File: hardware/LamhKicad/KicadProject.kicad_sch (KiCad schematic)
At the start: 45 parts, among them J1 JTAG-10 PIN, J2 436500303, J3 436500303, J4 436500303, J5 ESQ-110-X-X-D, J6 436500303, U1 TJA1051T-3, U2 PCA9685PW_112, U3 TLV70433DBVT, U4 STM32F072C8Tx

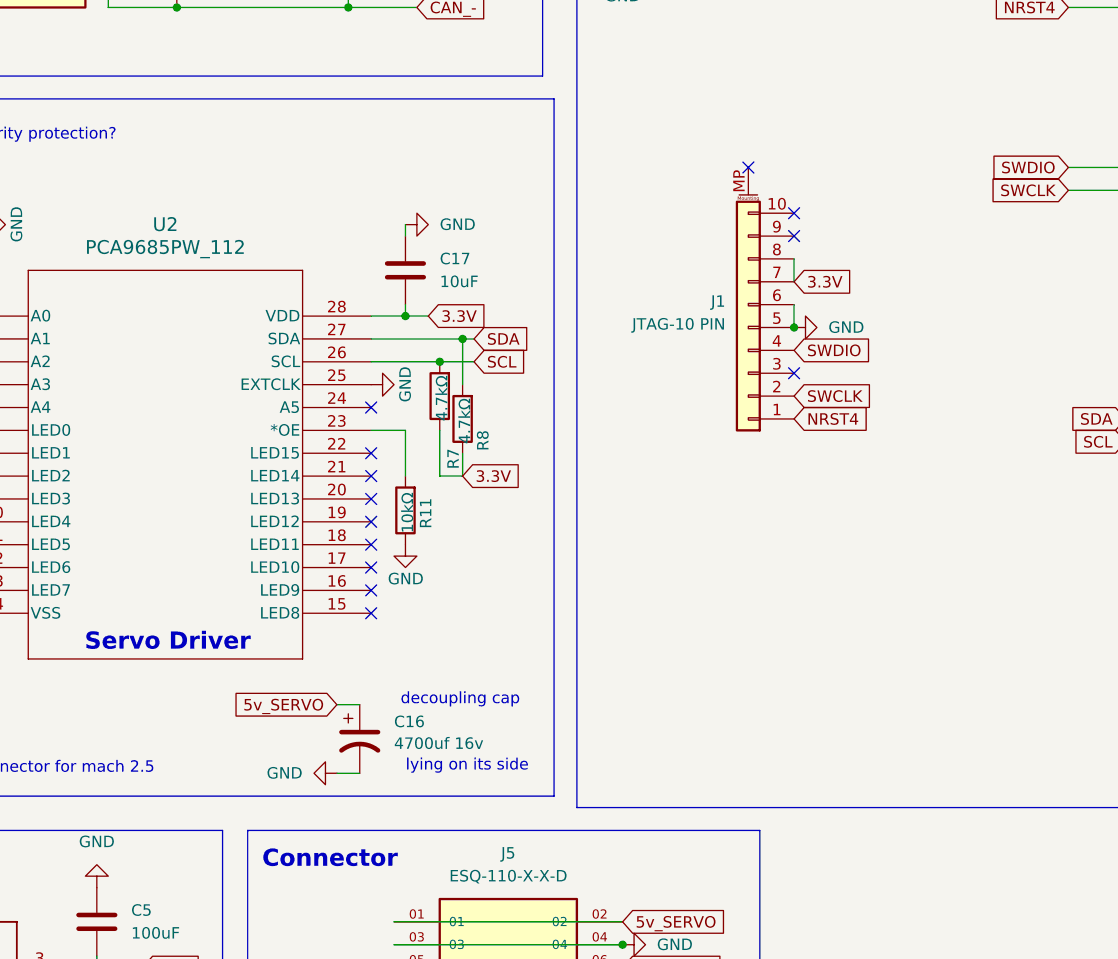
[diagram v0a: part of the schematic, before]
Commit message: ready to route
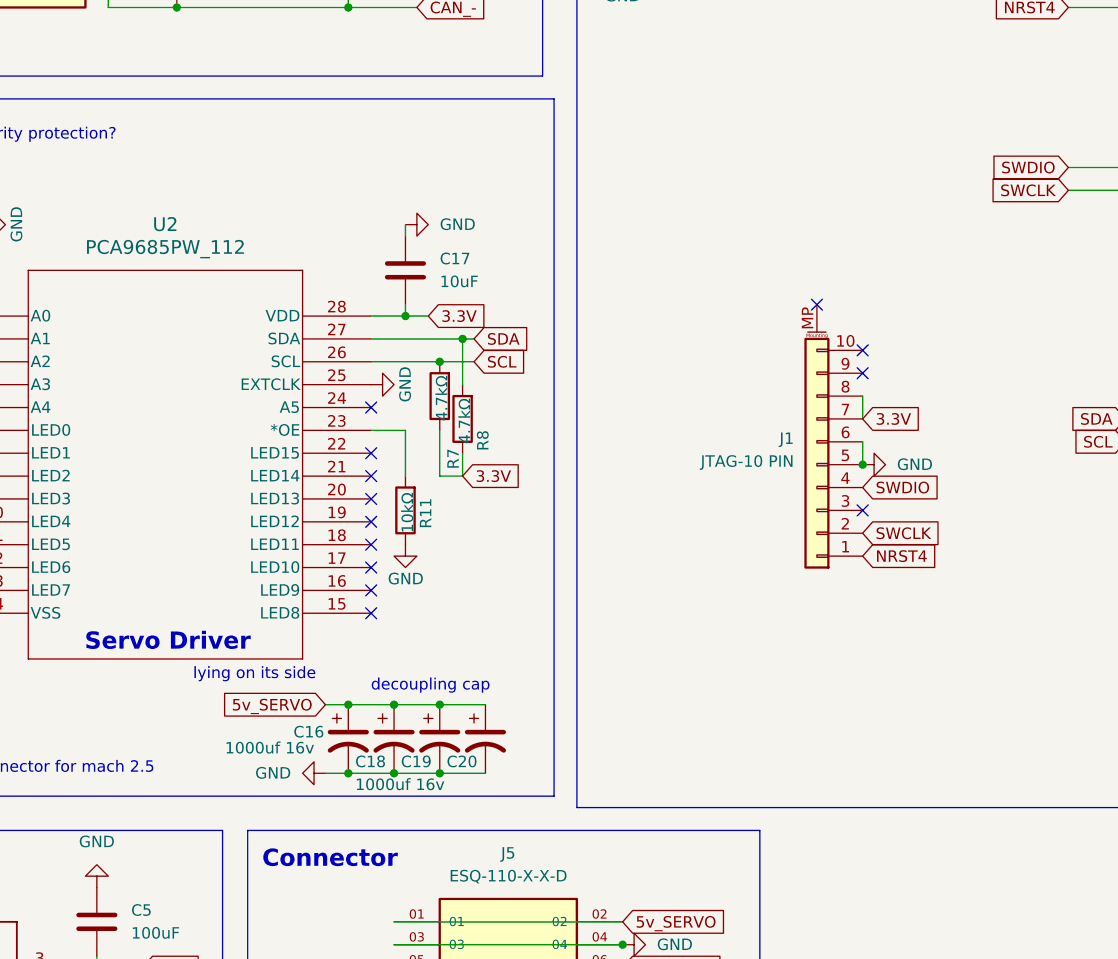
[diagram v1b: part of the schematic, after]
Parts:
- added C18, C19, C20: 1000uf 16v, Capacitor_THT:CP_Radial_D10.0mm_P5.00mm, symbol Device:C_Polarized_US
- C16: value 4700uf 16v -> 1000uf 16v; footprint (none) -> Capacitor_THT:CP_Radial_D10.0mm_P5.00mm
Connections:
- net 5v_SERVO: now also C18.1, C19.1, C20.1
- net GND: now also C18.2, C19.2, C20.2
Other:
- moved on the sheet: C16, J1

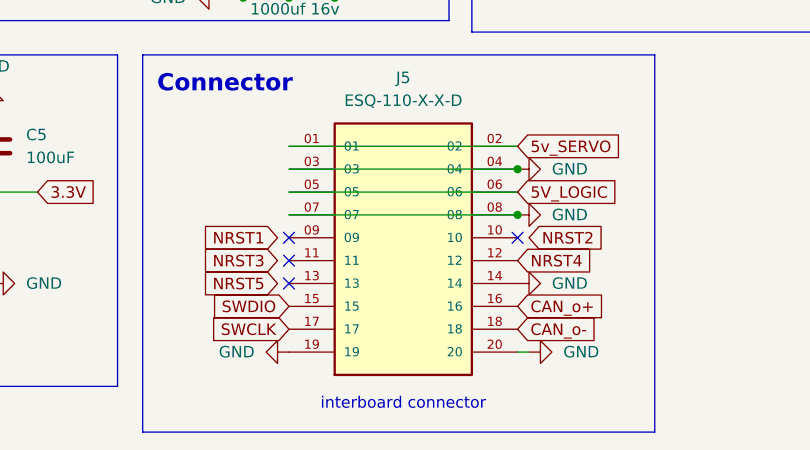
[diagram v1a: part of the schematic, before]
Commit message: fixed the connector
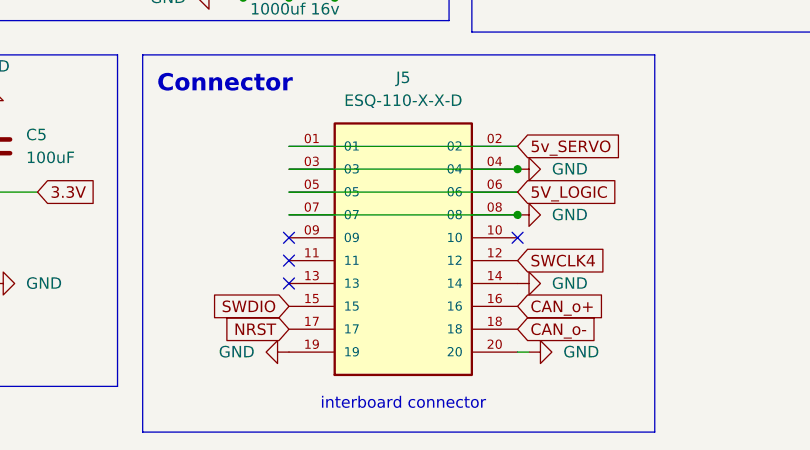
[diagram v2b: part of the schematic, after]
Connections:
- net NRST4: no longer J5.12
- net SWCLK: no longer J5.17
- new net NRST: J5.17
- new net SWCLK4: J5.12
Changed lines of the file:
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@@
-		)
-	)
-	(global_label "NRST2"
-		(shape input)
-		(at 195.58 198.12 0)
-		(fields_autoplaced yes)
-		(effects
-			(font
-				(size 1.27 1.27)
-			)
-			(justify left)
-		)
-		(property "Intersheetrefs" "${INTERSHEET_REFS}"
-			(at 204.5523 198.12 0)
-			(effects
-				(font
-					(size 1.27 1.27)
-				)
-				(justify left)
-				(hide yes)
-			)
 		)
 	)
@@
 		)
 	)
-	(global_label "NRST3"
-		(shape input)
-		(at 167.64 200.66 180)
-		(fields_autoplaced yes)
-		(effects
-			(font
-				(size 1.27 1.27)
-			)
-			(justify right)
-		)
-		(property "Intersheetrefs" "${INTERSHEET_REFS}"
-			(at 158.6677 200.66 0)
-			(effects
-				(font
-					(size 1.27 1.27)
-				)
-				(justify right)
-				(hide yes)
-			)
-		)
-	)
 	(global_label "3.3V"
 		(shape input)
@@
 		)
 	)
-	(global_label "NRST5"
-		(shape input)
-		(at 167.64 203.2 180)
-		(fields_autoplaced yes)
-		(effects
-			(font
-				(size 1.27 1.27)
-			)
-			(justify right)
-		)
-		(property "Intersheetrefs" "${INTERSHEET_REFS}"
-			(at 158.6677 203.2 0)
-			(effects
-				(font
-					(size 1.27 1.27)
-				)
-				(justify right)
-				(hide yes)
-			)
-		)
-	)
 	(global_label "MOSI"
 		(shape input)
@@
 		)
 	)
+	(global_label "NRST"
+		(shape input)
+		(at 168.91 208.28 180)
+		(fields_autoplaced yes)
+		(effects
+			(font
+				(size 1.27 1.27)
+			)
+			(justify right)
+		)
+		(property "Intersheetrefs" "${INTERSHEET_REFS}"
+			(at 161.1472 208.28 0)
+			(effects
+				(font
+					(size 1.27 1.27)
+				)
+				(justify right)
+				(hide yes)
+			)
+		)
+	)
 	(global_label "SWCLK"
 		(shape input)
-		(at 168.91 208.28 180)
-		(fields_autoplaced yes)
-		(effects
-			(font
-				(size 1.27 1.27)
-			)
-			(justify right)
-		)
-		(property "Intersheetrefs" "${INTERSHEET_REFS}"
-			(at 159.6958 208.28 0)
-			(effects
-				(font
-					(size 1.27 1.27)
-				)
-				(justify right)
-				(hide yes)
-			)
-		)
-	)
-	(global_label "SWCLK"
-		(shape input)
 		(at 243.84 106.68 180)
 		(fields_autoplaced yes)
@@
 		)
 	)
-	(global_label "NRST1"
-		(shape input)
-		(at 167.64 198.12 180)
-		(fields_autoplaced yes)
-		(effects
-			(font
-				(size 1.27 1.27)
-			)
-			(justify right)
-		)
-		(property "Intersheetrefs" "${INTERSHEET_REFS}"
-			(at 158.6677 198.12 0)
-			(effects
-				(font
-					(size 1.27 1.27)
-				)
-				(justify right)
-				(hide yes)
-			)
-		)
-	)
 	(global_label "3.3V"
 		(shape input)
@@
 		)
 	)
-	(global_label "NRST4"
+	(global_label "SWCLK4"
 		(shape input)
 		(at 194.31 200.66 0)
@@
 		)
 		(property "Intersheetrefs" "${INTERSHEET_REFS}"
-			(at 203.2823 200.66 0)
-			(effects
-				(font
+			(at 204.7337 200.66 0)
+			(effects
+				(font
